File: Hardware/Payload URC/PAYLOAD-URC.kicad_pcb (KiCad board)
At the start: 4 copper layers, 87 x 54 mm, 94 parts, among them J1 VG2080001H, J18 Conn_01x02, J2 Conn_01x02, J20 Conn_01x02, J3 Conn_01x02, J4 Conn_01x02, J5 Conn_01x03, J6 ST-Link-Conn-SM, J7 Conn_01x02, J8 Conn_01x03, Q1 AO3400A, Q2 AO3400A, Q5 AO3400A, Q6 AO3400A, SW2 SW_Oval, U10 THVD1500DR, U3 TPD4E05U06DQAR, U4 TLV75533PDBV, U5 ADS1115IDGS, U6 STM32C542CCT6, U8 TPD4E05U06DQAR, U9 TPS7A20xxxDBV, Y1 XTAL3225 (16M, 9P)

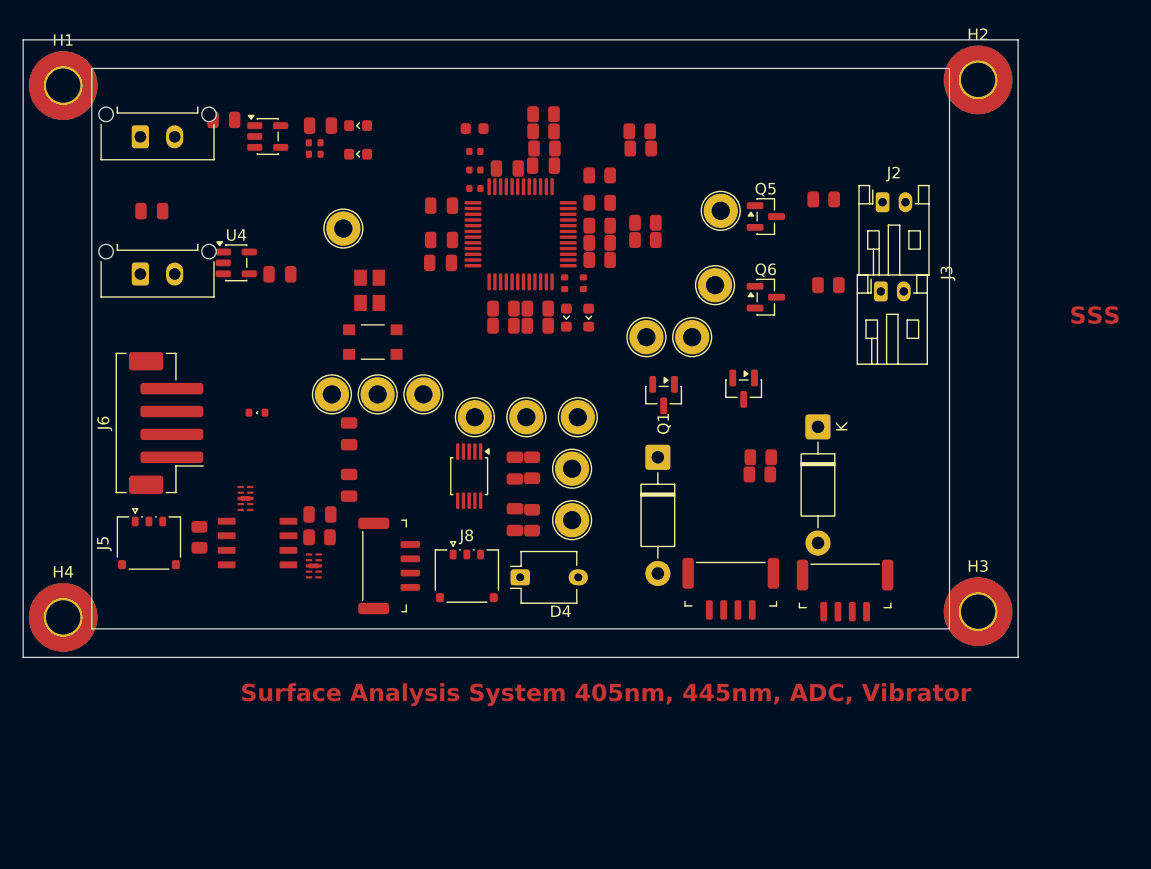
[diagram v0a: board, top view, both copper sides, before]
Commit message: Update
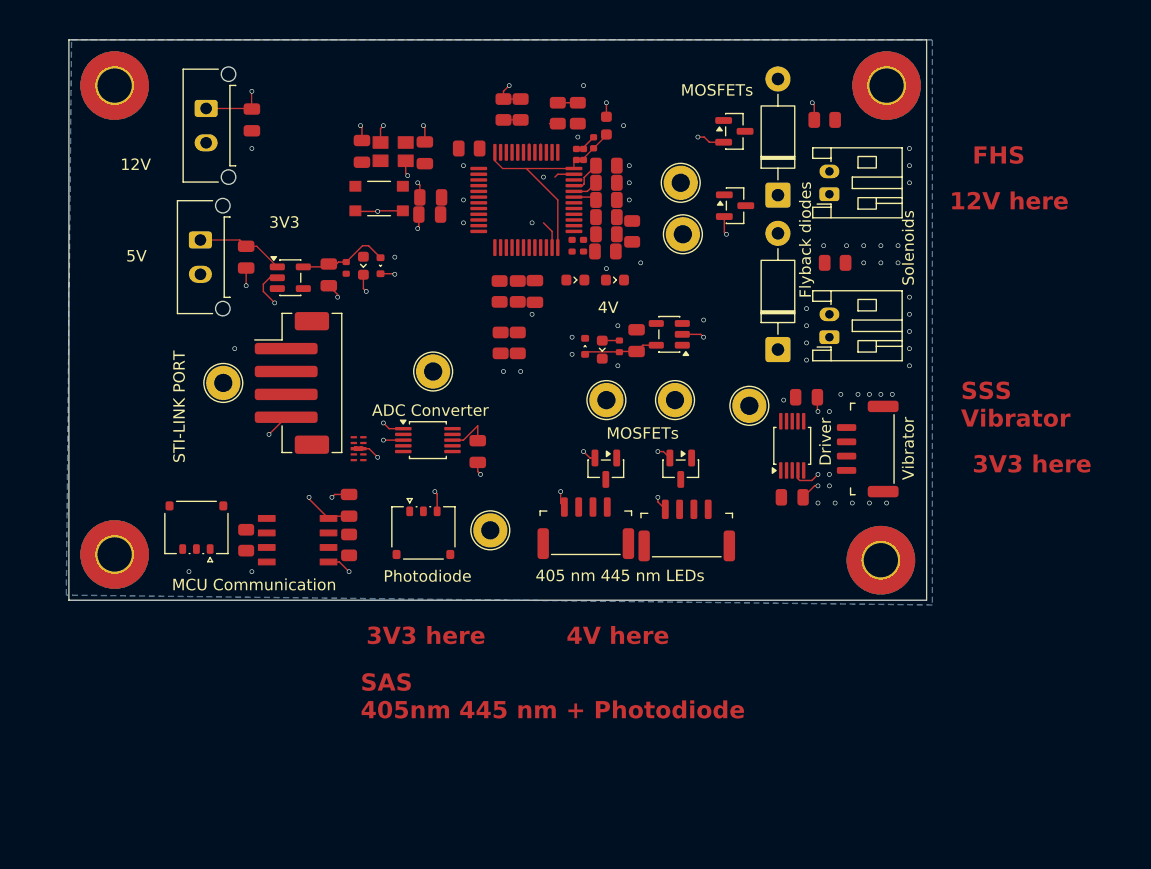
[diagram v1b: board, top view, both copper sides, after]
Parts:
- removed C17: 0.1u, SCRB_STD_Passives:C0805
- removed J18: Conn_01x02, SCRB_Connectors:JST-GH-SM04B-GHS-TB
- removed J5: Conn_01x03, Connector_Hirose:Hirose_DF57H-3P-1.2V_1x03_P1.2mm_Socket
- removed R21: 120, SCRB_STD_Passives:R0805
- removed R28, R29: 10, SCRB_STD_Passives:R0805
- removed R40: 10k, SCRB_STD_Passives:R0805
- removed R45: 6.6k, SCRB_STD_Passives:R0805
- removed TP19, TP20, TP26, TP36, TP37: TestPoint, TestPoint:TestPoint_Loop_D2.60mm_Drill1.6mm_Beaded
- removed U10: THVD1500DR, SCRB_TexasInstruments:D0008A
- removed U8: TPD4E05U06DQAR, SCRB_TexasInstruments:DQA0010A
- added J19: Conn_01x02, SCRB_Connectors:JST-GH-SM04B-GHS-TB, F.Cu at (83.2, 105.2)
- added J9: Conn_01x03, Connector_Hirose:Hirose_DF57H-3P-1.2V_1x03_P1.2mm_Socket, F.Cu at (69.0, 105.6)
- added R22: 120, SCRB_STD_Passives:R0805, F.Cu at (62.5, 106.7)
- added U1: DRV2605LDGS, Package_SO:TSSOP-10_3x3mm_P0.5mm, F.Cu at (101.2, 98.0)
- added U11: THVD1500DR, SCRB_TexasInstruments:D0008A, F.Cu at (58.0, 106.2)
- C19: value 4.2p -> 0.1u
- D4: value BPW34 -> TVS_SOD523; footprint OptoDevice:Osram_DIL2_4.3x4.65mm_P5.08mm -> SCRB_STD_Actives:SOD-523
- H1, H2, H3, H4: value MountingHole -> MH2.5
- R44: value 1M -> 10k
- moved J1 43.1 mm to (107.8, 98.3), turned to 90 degrees
- moved C20 40.1 mm to (102.5, 93.8), turned to 180 degrees
- moved U9 39.1 mm to (90.5, 88.2), turned to 180 degrees
- moved C21 38.8 mm to (101.2, 102.5), turned to 0 degrees
- moved TP35 36.5 mm to (97.5, 94.5)
- moved C11 33.4 mm to (87.6, 88.8), turned to 90 degrees
- moved R4 32.0 mm to (86.1, 89.3), turned to 90 degrees
- moved LD4 29.0 mm to (84.6, 89.6), turned to 90 degrees
- moved R44 25.1 mm to (53.5, 106.2), turned to 90 degrees
- moved J8 24.0 mm to (49.1, 105.1), turned to 180 degrees
- moved D4 21.0 mm to (83.1, 89.3), turned to -90 degrees
- moved D8 20.6 mm to (100.0, 76.1), turned to 90 degrees
- moved C2 18.2 mm to (60.7, 83.0), turned to -90 degrees
- moved TP2 17.1 mm to (51.5, 92.5)
- moved D3 16.8 mm to (65.2, 82.2), turned to 90 degrees
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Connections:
- C19 pad 1: Net-(D4-K) -> /5V
- C19 pad 2: Net-(C19-Pad2) -> GND
- D4 pad 1: Net-(D4-K) -> GND
- D4 pad 2: GND -> /4V
- J8 pad 1: Net-(J8-Pin_1) -> /JTCK/SWCLK
- J8 pad 2: Net-(J8-Pin_2) -> /ESD_protection/RS485A
- R44 pad 1: Net-(D4-K) -> GND
- R44 pad 2: Net-(C19-Pad2) -> Net-(U11-DE)
- U3 pad 4: unconnected-(U3-D3-Pad4) -> /ESD_protection/RS485A
- U3 pad 7: unconnected-(U3-NC-Pad7) -> /ESD_protection/RS485A
- U3 pad 9: unconnected-(U3-NC-Pad9) -> /JTCK/SWCLK
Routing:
- net GND: track 0.00 -> 57.9 mm, vias 2 -> 86
- net /3V3: track 0.00 -> 34.3 mm, vias 4 -> 9
- net /5V: track 0.00 -> 15.0 mm, vias 0 -> 2
- net /4V: track 0.00 -> 9.38 mm, vias 0 -> 3
- net /12V: track 0.00 -> 7.16 mm, vias 0 -> 3
- net /I2C1_SDA: track 0.00 -> 2.98 mm
- net /I2C1_SCL: track 0.00 -> 2.24 mm
- net /GPIO: track 0.00 -> 2.03 mm
- net /UART4_TX: track 0.00 -> 1.85 mm
- net Net-(LD4-A): track 0.00 -> 1.50 mm
- net /I2C1_SCL_1: track 0.00 -> 1.46 mm
- net /I2C1_SDA_1: track 0.00 -> 0.74 mm
- net /PB14_GPIO: track 0.00 -> 0.68 mm
- added copper zone on In2.Cu, net /12V
- added copper zone on In2.Cu, net /4V
- added copper zone on In2.Cu, net /5V
- added copper zone on B.Cu, net GND
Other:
- board size 87 x 54 mm -> 75 x 49 mm
- board text added: "12V"
- board text added: "12V here"
- board text added: "3V3"
- board text added: "3V3 here"
- board text added: "405 nm 445 nm LEDs"
- board text added: "4V"
- board text added: "4V here"
- board text added: "5V"
- board text added: "ADC Converter"
- board text added: "Driver"
- board text added: "FHS"
- board text added: "Flyback diodes"
- board text added: "MCU Communication"
- board text added: "MOSFETs"
- board text added: "Photodiode"
- board text added: "SAS 405nm 445 nm + Photodiode"
- board text added: "SSS Vibrator"
- board text added: "STI-LINK PORT"
- board text added: "Solenoids"
- board text added: "Vibrator"
- board text removed: "SSS"
- board text removed: "Surface Analysis System 405nm, 445nm, ADC, Vibrator"
